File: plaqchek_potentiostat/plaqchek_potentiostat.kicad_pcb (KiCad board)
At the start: 2 copper layers, 46 x 59.8 mm, 57 parts, among them J1 Conn_01x03, J2 Conn_01x03, J3 Conn_01x02, SW2 SW_SPDT, U1 TL082, U3 TL082, U4 TL082, U5 TPS7A2050PDBVR, U6 MC79M05_TO252

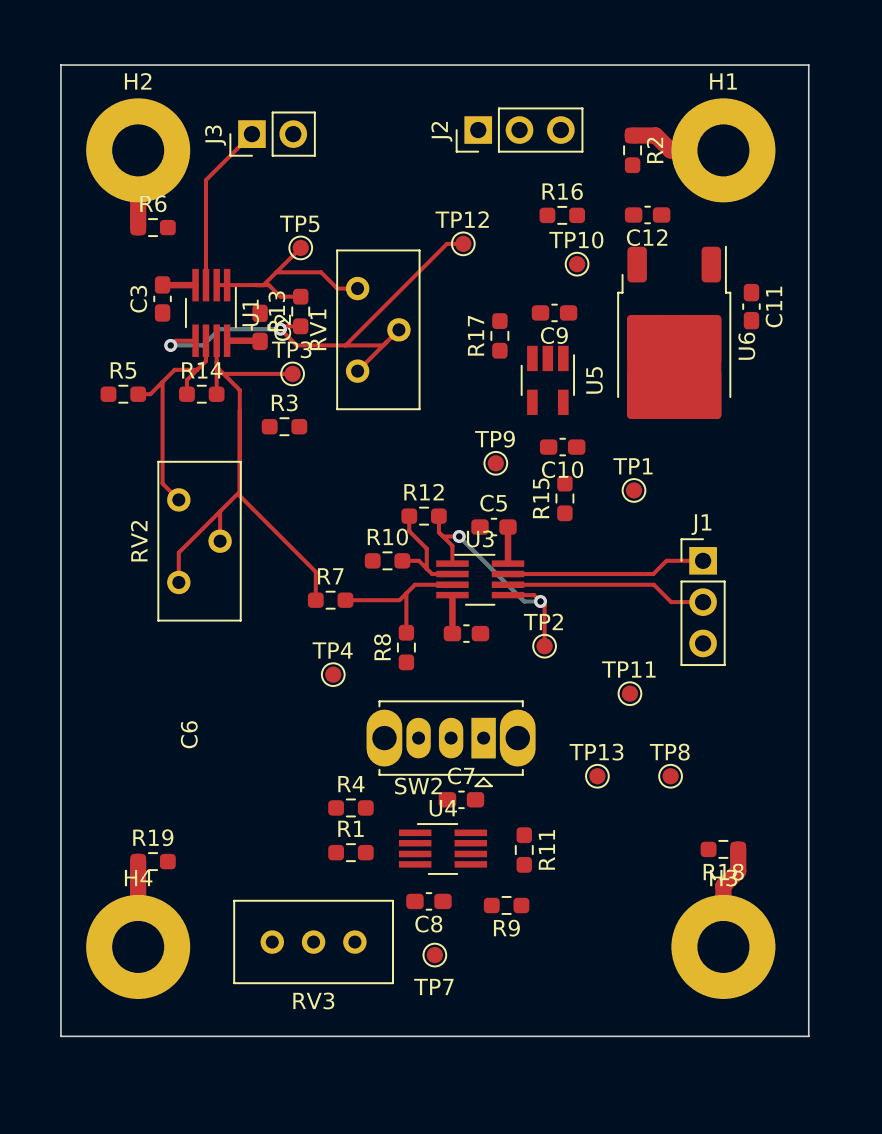
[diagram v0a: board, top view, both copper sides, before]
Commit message: more routing
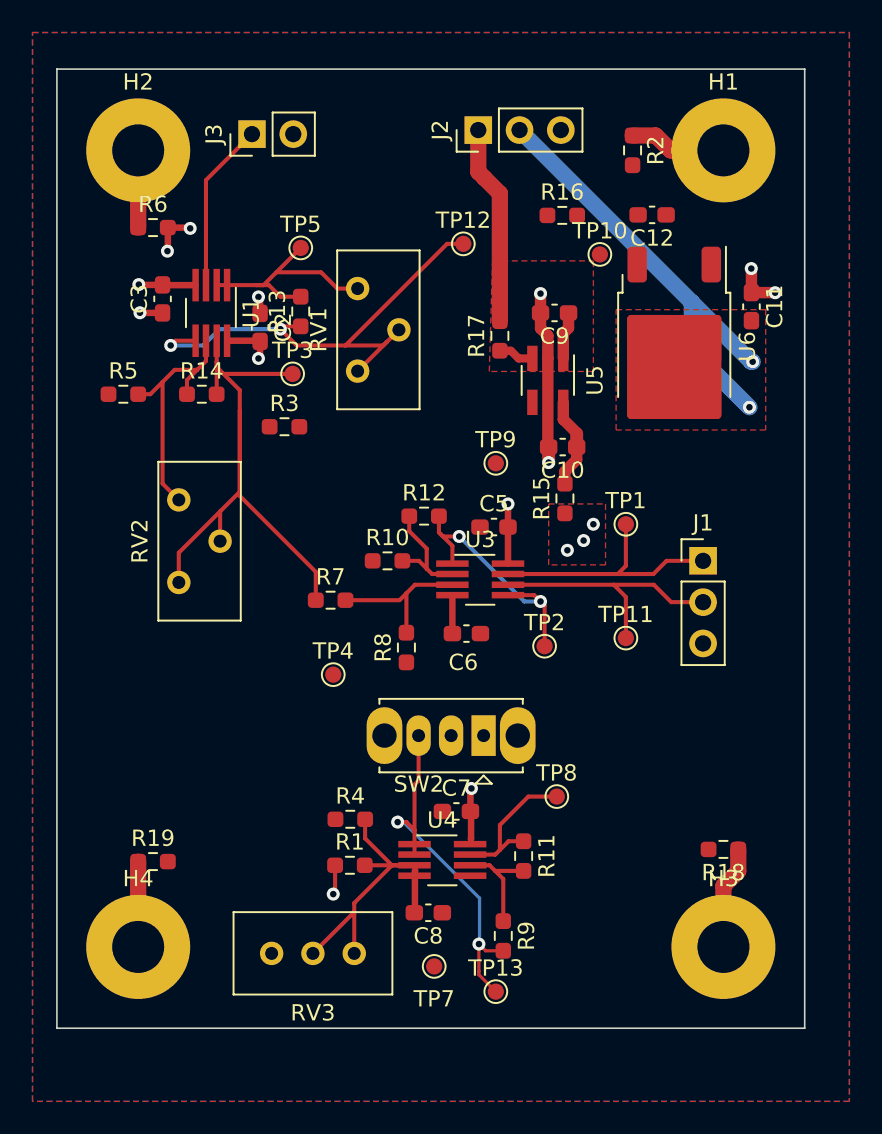
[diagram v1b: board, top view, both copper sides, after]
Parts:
- moved TP13 14.7 mm to (171.0, 143.8)
- moved TP8 7.11 mm to (174.8, 131.8)
- moved TP11 3.43 mm to (179.0, 122.0)
- moved TP1 2.14 mm to (179.0, 115.0)
- moved R9 1.88 mm to (171.5, 140.3), turned to -90 degrees
- moved TP10 1.52 mm to (177.4, 98.4)
- moved C7 0.78 mm to (168.6, 132.7)
- moved R1 0.78 mm to (162.0, 136.0)
- moved C8 0.70 mm to (166.8, 138.9)
- moved R4 0.70 mm to (162.0, 133.1)
- moved RV3 0.70 mm to (157.2, 141.4)
- moved U4 0.70 mm to (167.7, 135.6)
- moved TP7 0.70 mm to (167.2, 142.2)
- moved R11 0.37 mm to (172.7, 135.4)
- moved C12 0.28 mm to (180.6, 96.0)
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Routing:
- net -6V5: track 0.00 -> 28.2 mm, vias 0 -> 2
- net /VBIAS_POT_P: track 0.00 -> 23.3 mm, vias 0 -> 2
- net GND: track 0.00 -> 18.8 mm, vias 0 -> 8
- net Net-(U4A-+): track 0.00 -> 16.9 mm
- net +6V: track 0.00 -> 15.2 mm
- net /VBIAS_POT_N: track 0.00 -> 9.38 mm
- net +5VA: track 4.30 -> 12.1 mm, vias 0 -> 7
- net Net-(U4B--): track 0.00 -> 6.73 mm
- net Net-(U5-OUT): track 0.00 -> 5.63 mm
- net -5VA: track 4.40 -> 8.16 mm, vias 0 -> 1
- net /REF_ELEC: track 12.7 -> 16.3 mm
- net /WORKING_ELEC: track 12.3 -> 15.6 mm
- net Net-(U5-EN): track 0.00 -> 2.20 mm
- added copper zone on F.Cu, net +5VA
- added copper zone on In2.Cu, net +5VA
- added copper zone on F.Cu, net +6V
- added copper zone on In2.Cu, net -5VA
- added copper zone on F.Cu, net -6V5
- added copper zone on B.Cu, net GND
- added copper zone on F.Cu, net GND
- added copper zone on In1.Cu, net GND
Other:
- board size 46 x 59.8 mm -> 46 x 59 mm
- copper layers 2 -> 4
